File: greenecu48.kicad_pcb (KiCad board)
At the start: 4 copper layers, 128 x 110.6 mm, 75 parts, among them J4 USB_B_Mini, M1 Module-power_12and5V-0.1, M3 Module-knock-0.2, M4 Module-ign8-0.2, M5 Module-wbo-0.5, M6 Module-can-0.1, M7 Module-ign8-0.2, M8 Module-vr-max9924-0.1, M9 Module-mega-mcu144-0.7, Q11 ISL9V3040D3ST, Q12 ISL9V3040D3ST, Q14 ISL9V3040D3ST, Q9 ISL9V3040D3ST, Q901 ISL9V3040D3ST, Q902 ISL9V3040D3ST, Q903 ISL9V3040D3ST, Q904 ISL9V3040D3ST, Q905 ISL9V3040D3ST, Q906 ISL9V3040D3ST, Q911 ISL9V3040D3ST, Q912 ISL9V3040D3ST, Q913 ISL9V3040D3ST, Q914 ISL9V3040D3ST, Q915 ISL9V3040D3ST, Q916 ISL9V3040D3ST, U1 molex_48pin_MRE, U2 MAX31855KASA

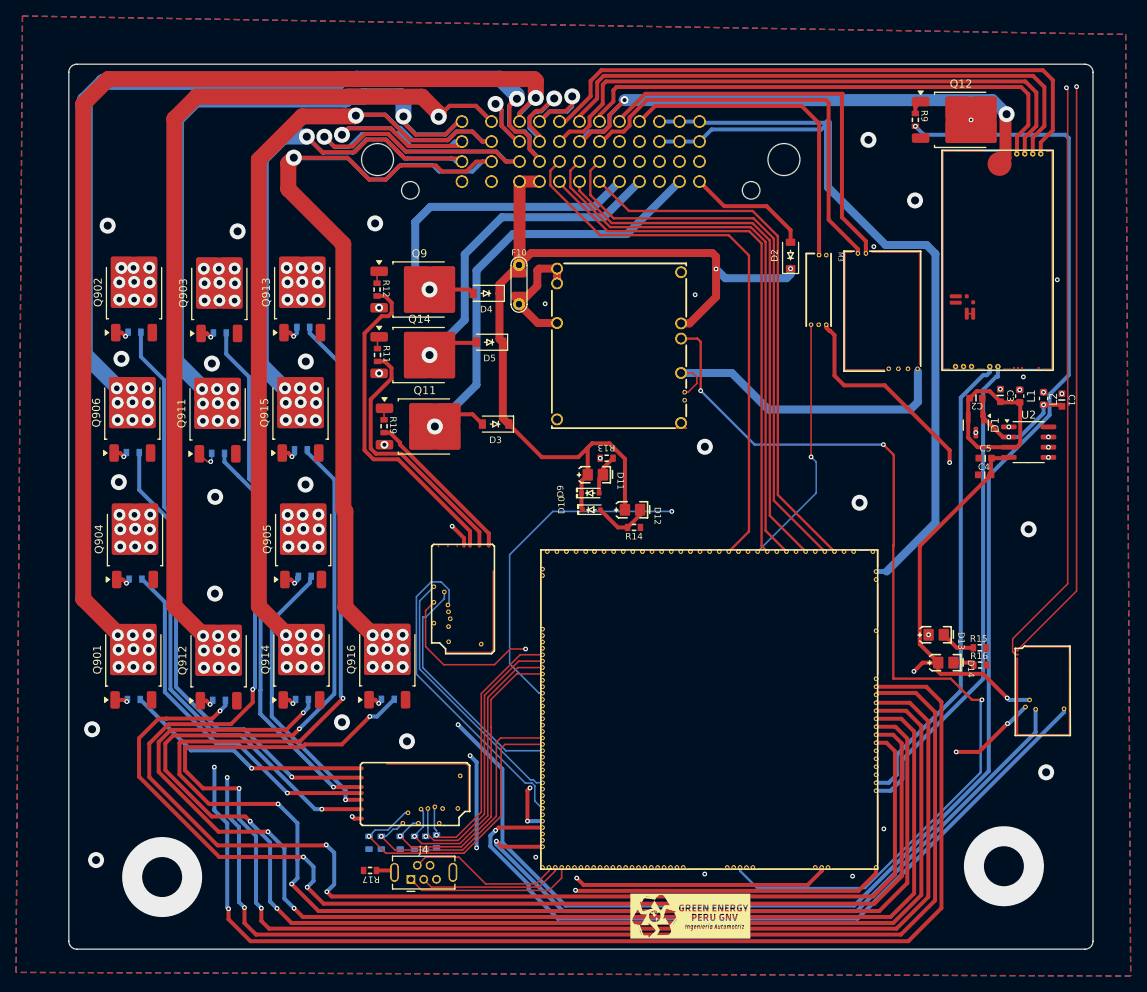
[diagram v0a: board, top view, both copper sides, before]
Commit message: ok
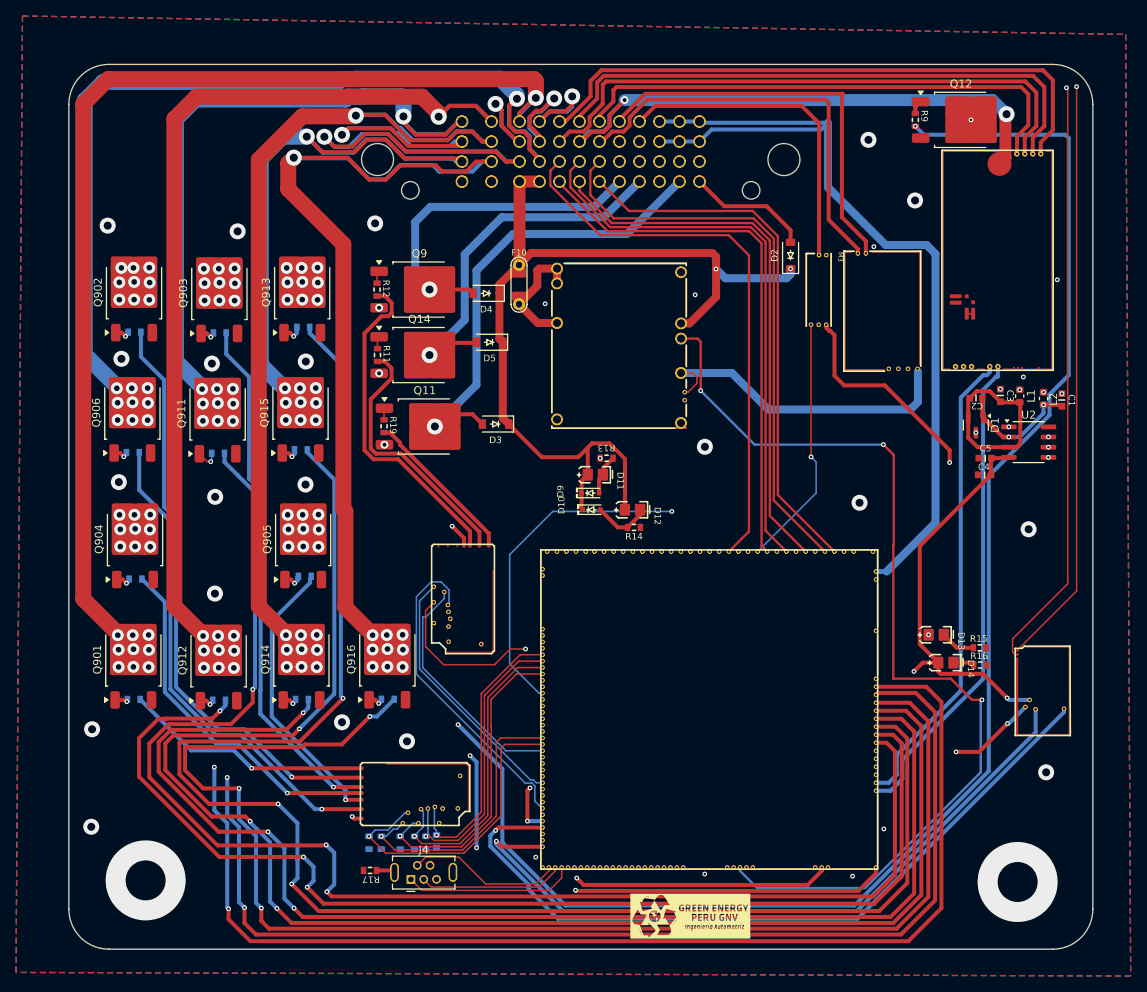
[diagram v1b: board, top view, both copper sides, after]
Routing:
- net GND: vias 37 -> 39
- net (no net): vias 2 -> 0
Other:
- outline, holes or cut-outs redrawn
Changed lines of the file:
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@@
 	)
 	(gr_line
-		(start 209.11 24.06)
-		(end 209.11 132.68)
+		(start 209.09 28.08)
+		(end 209.09 128.68)
 		(stroke
 			(width 0.05)
@@
 		(layer "Edge.Cuts")
 	)
-	(gr_arc
-		(start 209.11 132.68)
-		(mid 208.817107 133.387107)
-		(end 208.11 133.68)
+	(gr_line
+		(start 204.09 133.68)
+		(end 86.09 133.68)
 		(stroke
 			(width 0.05)
@@
 	)
 	(gr_arc
-		(start 208.11 23.06)
-		(mid 208.817107 23.352893)
-		(end 209.11 24.06)
+		(start 81.09 28.08)
+		(mid 82.554466 24.544466)
+		(end 86.09 23.08)
 		(stroke
 			(width 0.05)
@@
 		(layer "Edge.Cuts")
 	)
-	(gr_line
-		(start 208.11 133.68)
-		(end 82.09 133.68)
+	(gr_arc
+		(start 204.09 23.08)
+		(mid 207.625534 24.544466)
+		(end 209.09 28.08)
 		(stroke
 			(width 0.05)
@@
 		(layer "Edge.Cuts")
 	)
-	(gr_line
-		(start 82.09 23.06)
-		(end 208.11 23.06)
+	(gr_arc
+		(start 86.09 133.68)
+		(mid 82.554466 132.215534)
+		(end 81.09 128.68)
 		(stroke
 			(width 0.05)
@@
 		(layer "Edge.Cuts")
 	)
-	(gr_line
-		(start 81.09 132.68)
-		(end 81.09 24.06)
+	(gr_arc
+		(start 209.09 128.68)
+		(mid 207.625534 132.215534)
+		(end 204.09 133.68)
 		(stroke
 			(width 0.05)
@@
 		(layer "Edge.Cuts")
 	)
-	(gr_arc
-		(start 82.09 133.68)
-		(mid 81.382893 133.387107)
-		(end 81.09 132.68)
+	(gr_line
+		(start 86.09 23.08)
+		(end 204.09 23.08)
 		(stroke
 			(width 0.05)
@@
 		(layer "Edge.Cuts")
 	)
-	(gr_arc
-		(start 81.09 24.06)
-		(mid 81.382893 23.352893)
-		(end 82.09 23.06)
+	(gr_line
+		(start 81.09 128.68)
+		(end 81.09 28.08)
 		(stroke
 			(width 0.05)
@@
 		(layer "Edge.Cuts")
 	)
-	(via
-		(at 197.973923 123.308121)
-		(size 10)
-		(drill 5)
-		(layers "F.Cu" "B.Cu")
-		(net 0)
-	)
-	(via
-		(at 92.754932 124.66164)
-		(size 10)
-		(drill 5)
-		(layers "F.Cu" "B.Cu")
-		(net 0)
-	)
 	(segment
 		(start 138.413 117.674997)
@@
 	)
 	(via
-		(at 84.493 122.538)
+		(at 83.89 118.38)
 		(size 2)
 		(drill 1)
@@
 	)
 	(via
+		(at 199.69 125.28)
+		(size 10)
+		(drill 5)
+		(layers "F.Cu" "B.Cu")
+		(net 4)
+	)
+	(via
 		(at 194.465 69.109)
 		(size 0.6)
@@
 		(net 4)
 	)
+	(via
+		(at 90.69 125.08)
+		(size 10)
+		(drill 5)
+		(layers "F.Cu" "B.Cu")
+		(net 4)
+	)
